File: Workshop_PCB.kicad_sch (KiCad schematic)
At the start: 23 parts, among them J1 Conn_01x04, J2 USB_C_Receptacle_USB2.0_16P, J3 Conn_01x22, J4 Conn_01x22, SW1 SW_Push, U1 STM32F042C6Tx, U2 AMS1117-3.3, U3 USBLC6-2SC6

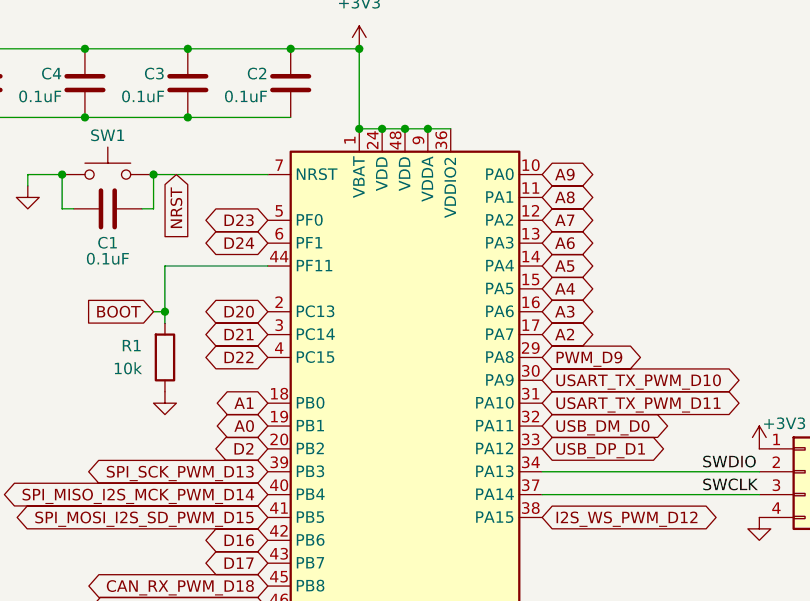
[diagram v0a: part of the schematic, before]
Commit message: Start tracing board
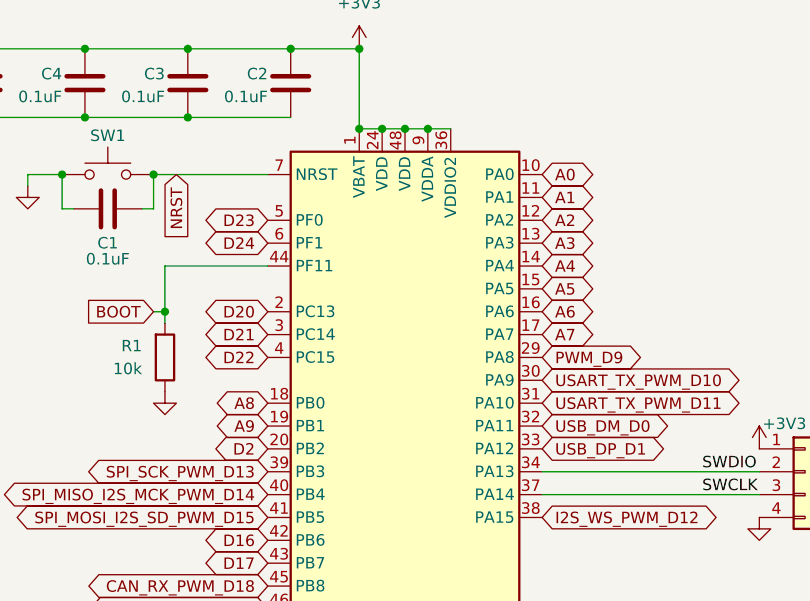
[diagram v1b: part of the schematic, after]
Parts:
- J1: footprint Connector_PinSocket_2.54mm:PinSocket_1x04_P2.54mm_Horizontal -> Connector_PinSocket_2.54mm:PinSocket_1x04_P2.54mm_Vertical
- J3, J4: LCSC C2765186 -> (none)
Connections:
- net A0: now also U1.10 (PA0); no longer U1.19 (PB1)
- net A1: now also U1.11 (PA1); no longer U1.18 (PB0)
- net A2: now also U1.12 (PA2); no longer U1.17 (PA7)
- net A3: now also U1.13 (PA3); no longer U1.16 (PA6)
- net A4: now also U1.14 (PA4); no longer U1.15 (PA5)
- net A5: now also U1.15 (PA5); no longer U1.14 (PA4)
- net A6: now also U1.16 (PA6); no longer U1.13 (PA3)
- net A7: now also U1.17 (PA7); no longer U1.12 (PA2)
- net A8: now also U1.18 (PB0); no longer U1.11 (PA1)
- net A9: now also U1.19 (PB1); no longer U1.10 (PA0)
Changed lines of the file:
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@@
 		)
 	)
-	(global_label "A8"
+	(global_label "A1"
 		(shape bidirectional)
 		(at 113.03 53.34 0)
@@
 		)
 	)
-	(global_label "A6"
+	(global_label "A3"
 		(shape bidirectional)
 		(at 113.03 58.42 0)
@@
 		)
 	)
-	(global_label "A2"
+	(global_label "A7"
 		(shape bidirectional)
 		(at 113.03 68.58 0)
@@
 		)
 	)
-	(global_label "A5"
+	(global_label "A4"
 		(shape bidirectional)
 		(at 113.03 60.96 0)
@@
 		)
 	)
-	(global_label "A9"
+	(global_label "A0"
 		(shape bidirectional)
 		(at 113.03 50.8 0)
@@
 		)
 	)
-	(global_label "A1"
+	(global_label "A8"
 		(shape bidirectional)
 		(at 82.55 76.2 180)
@@
 		)
 	)
-	(global_label "A3"
+	(global_label "A6"
 		(shape bidirectional)
 		(at 113.03 66.04 0)
@@
 		)
 	)
-	(global_label "A4"
+	(global_label "A5"
 		(shape bidirectional)
 		(at 113.03 63.5 0)
@@
 		)
 	)
-	(global_label "A0"
+	(global_label "A9"
 		(shape bidirectional)
 		(at 82.55 78.74 180)
@@
 		)
 	)
-	(global_label "A7"
+	(global_label "A2"
 		(shape bidirectional)
 		(at 113.03 55.88 0)
@@
 			)
 		)
-		(property "Footprint" "Connector_PinSocket_2.54mm:PinSocket_1x04_P2.54mm_Horizontal"
+		(property "Footprint" "Connector_PinSocket_2.54mm:PinSocket_1x04_P2.54mm_Vertical"
 			(at 142.24 83.82 0)
 			(effects
@@
 			)
 		)
-		(property "LCSC" "C2765186"
+		(property "LCSC" ""
 			(at 186.69 123.19 0)
 			(effects
@@
 			)
 		)
-		(property "LCSC" "C2765186"
+		(property "LCSC" ""
 			(at 181.61 123.19 0)
 			(effects

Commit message: Finish PCB
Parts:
- J1: footprint Connector_PinSocket_2.54mm:PinSocket_1x04_P2.54mm_Vertical -> Connector_PinHeader_2.54mm:PinHeader_1x04_P2.54mm_Vertical
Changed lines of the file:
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@@
 			)
 		)
-		(property "Footprint" "Connector_PinSocket_2.54mm:PinSocket_1x04_P2.54mm_Vertical"
+		(property "Footprint" "Connector_PinHeader_2.54mm:PinHeader_1x04_P2.54mm_Vertical"
 			(at 142.24 83.82 0)
 			(effects
